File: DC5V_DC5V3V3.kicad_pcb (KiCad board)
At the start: 2 copper layers, 21.5 x 20 mm, 27 parts, among them J1 Vout1, J2 Vout2, Q1 BSS138, U1 LM1117-3.3

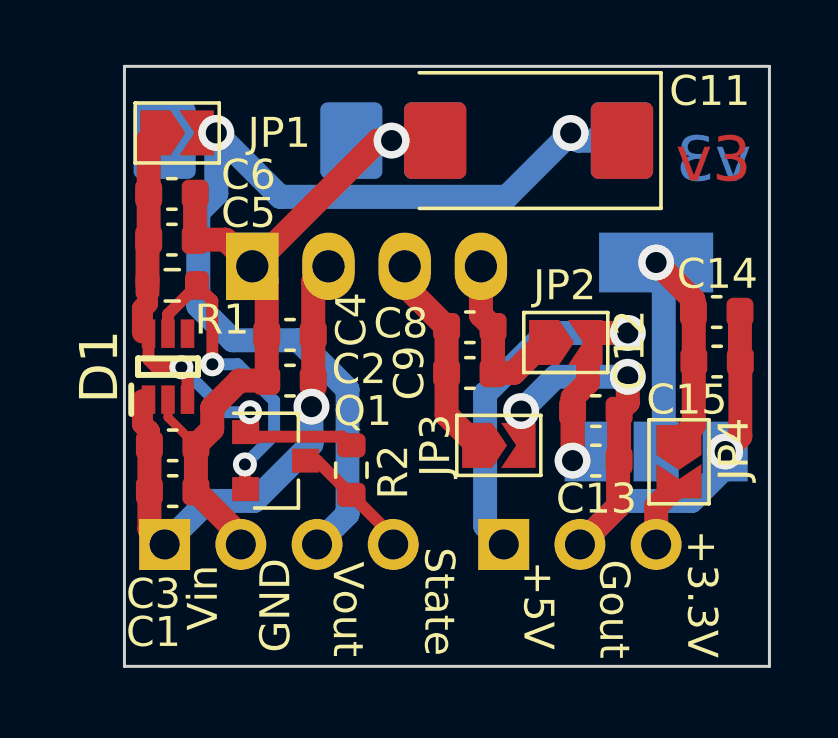
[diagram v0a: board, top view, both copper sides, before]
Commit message: Окончена трассировка печатной платы
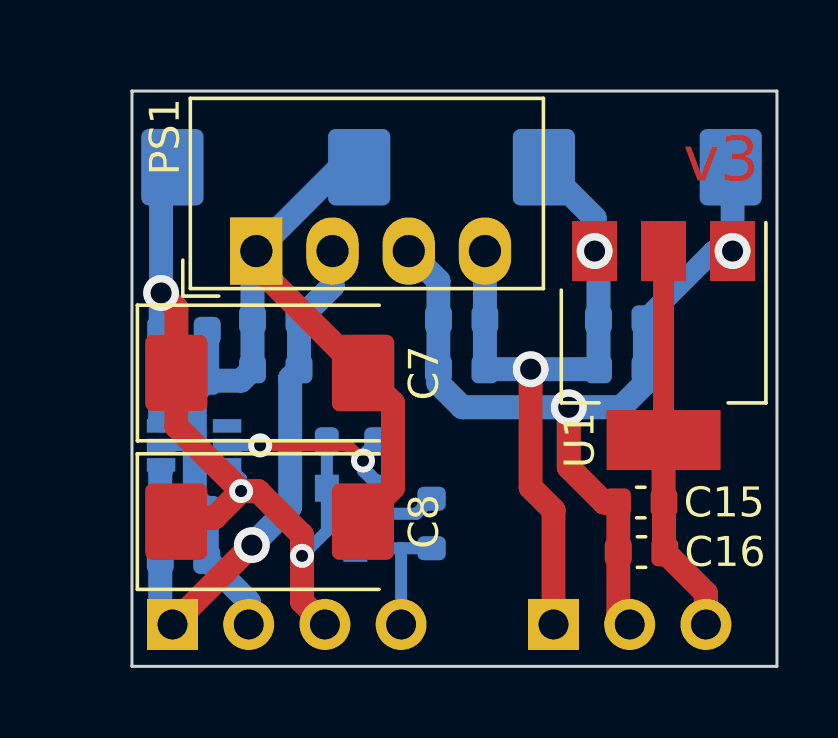
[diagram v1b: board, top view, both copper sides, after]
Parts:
- removed JP1: 5V_en, Jumper:SolderJumper-2_P1.3mm_Open_TrianglePad1.0x1.5mm
- removed JP2: 5VL_en, Jumper:SolderJumper-2_P1.3mm_Open_TrianglePad1.0x1.5mm
- removed JP3: N_en, Jumper:SolderJumper-2_P1.3mm_Open_TrianglePad1.0x1.5mm
- removed JP4: 3V3_en, Jumper:SolderJumper-2_P1.3mm_Open_TrianglePad1.0x1.5mm
- added C12: 470uF, Capacitor_Tantalum_SMD:CP_EIA-7343-15_Kemet-W, B.Cu at (106.1, 83.4)
- C1, C11, C2, C3, C4, C5, C6, D1, Q1, R1, R2: moved to B.Cu
- C10: renamed from C9; moved to B.Cu
- C13: renamed from C12; moved to B.Cu
- C14: renamed from C13; moved to B.Cu
- C7, PS1, U1: moved to F.Cu
- C8: renamed from C10; moved to F.Cu
- C9: renamed from C8; moved to B.Cu
- J1: footprint Connector_PinHeader_2.54mm:PinHeader_1x04_P2.54mm_Horizontal -> Modules:PinHeader_1x04_P2.54mm_Horizontal
- J2: footprint Connector_PinHeader_2.54mm:PinHeader_1x03_P2.54mm_Horizontal -> Modules:PinHeader_1x03_P2.54mm_Horizontal
- moved C8 15.4 mm to (93.8, 95.2), turned to 0 degrees
- moved C11 8.81 mm to (93.7, 83.4), turned to 0 degrees
- moved R1 7.93 mm to (96.6, 92.5)
- moved C7 7.76 mm to (93.8, 90.2)
- moved C15 6.84 mm to (106.2, 94.5), turned to 0 degrees
- moved C16 6.83 mm to (106.2, 96.2), turned to 0 degrees
- moved C5 4.72 mm to (91.0, 90.5)
- moved C6 4.59 mm to (91.0, 88.8)
- moved Q1 3.28 mm to (96.7, 95.1), turned to 270 degrees
- moved R2 3.21 mm to (99.2, 95.2)
- moved C13 3.17 mm to (105.6, 88.4)
- moved C14 3.17 mm to (105.6, 90.1)
- moved J2 3.14 mm to (103.3, 98.6)
- moved D1 2.76 mm to (91.3, 92.6), turned to 0 degrees
- moved J1 2.68 mm to (90.6, 98.6)
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- renumbered C14 to C15, C15 to C16
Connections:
- C10 pad 1: Net-(C8-Pad1) -> GND2
- C10 pad 2: Net-(C8-Pad2) -> +5VP
- C15 pad 2: Net-(C14-Pad2) -> +3.3VP
- C16 pad 2: Net-(C14-Pad2) -> +3.3VP
- C5 pad 2: /+5P0 -> +5P
- C6 pad 2: /+5P0 -> +5P
- C9 pad 1: Net-(C8-Pad1) -> GND2
- C9 pad 2: Net-(C8-Pad2) -> +5VP
- D1 pad 3: /+5P0 -> +5P
- D1 pad 4: Net-(D1-Pad4) -> (no net)
- D1 pad 6: /+5P0 -> +5P
- PS1 pad 3: Net-(C8-Pad1) -> GND2
- PS1 pad 4: Net-(C8-Pad2) -> +5VP
- Q1 pad 1: /+5P0 -> +5P
- R1 pad 1: /+5P0 -> +5P
- R2 pad 2: /+5P0 -> +5P
- U1 pad 2: Net-(C14-Pad2) -> +3.3VP
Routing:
- net /+5P0: track 17.6 -> 0.00 mm, vias 2 -> 0
- net Net-(C14-Pad2): track 13.2 -> 0.00 mm, vias 1 -> 0
- net +3.3VP: track 3.07 -> 13.0 mm
- net +5VP: track 16.5 -> 24.0 mm
- net Net-(C8-Pad1): track 6.97 -> 0.00 mm
- net GND1: track 26.5 -> 33.3 mm, vias 1 -> 0
- net GND2: track 23.4 -> 29.5 mm, vias 3 -> 2
- net Net-(C8-Pad2): track 5.84 -> 0.00 mm
- net Net-(D1-Pad5): track 10.8 -> 8.29 mm
- net +5V: track 17.8 -> 20.0 mm
- net +5P: track 35.8 -> 34.1 mm, vias 2 -> 3
- net /+5V_state: track 4.23 -> 5.08 mm
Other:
- board size 21.5 x 20 mm -> 21.5 x 19.2 mm
- board text added: "+5VP"
- board text added: "GND2"
- board text removed: "+5V"
- board text removed: "GND"
- board text removed: "Gout"
- board text removed: "State"
- board text removed: "Vin"
- board text removed: "Vout"
